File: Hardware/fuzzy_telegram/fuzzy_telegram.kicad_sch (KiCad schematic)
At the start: 1 part, among them U1 STM32MP157DAB1

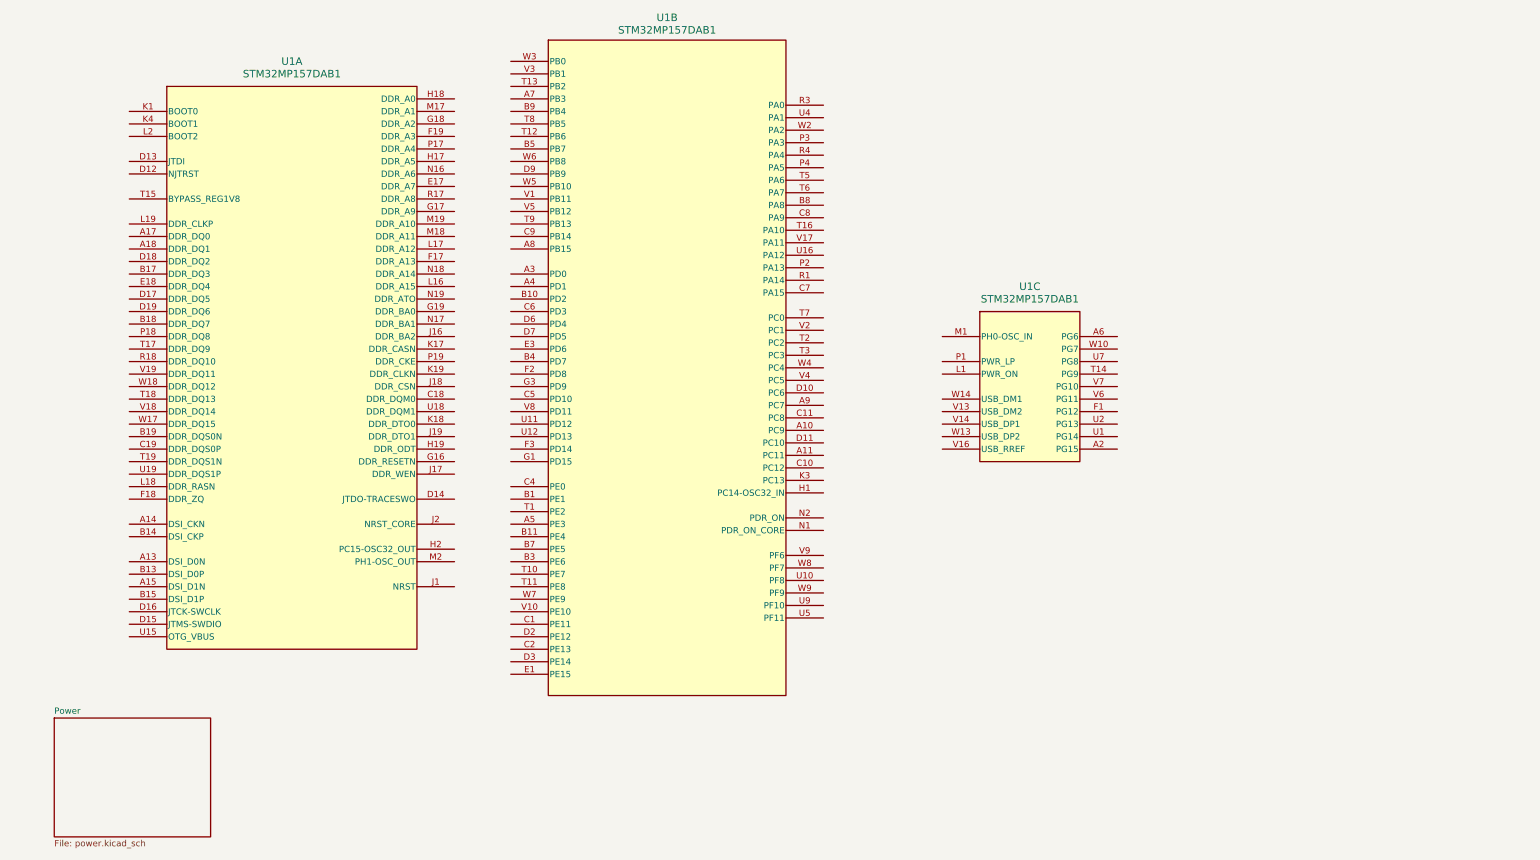
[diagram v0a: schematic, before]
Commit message: start on DDR3L schematic
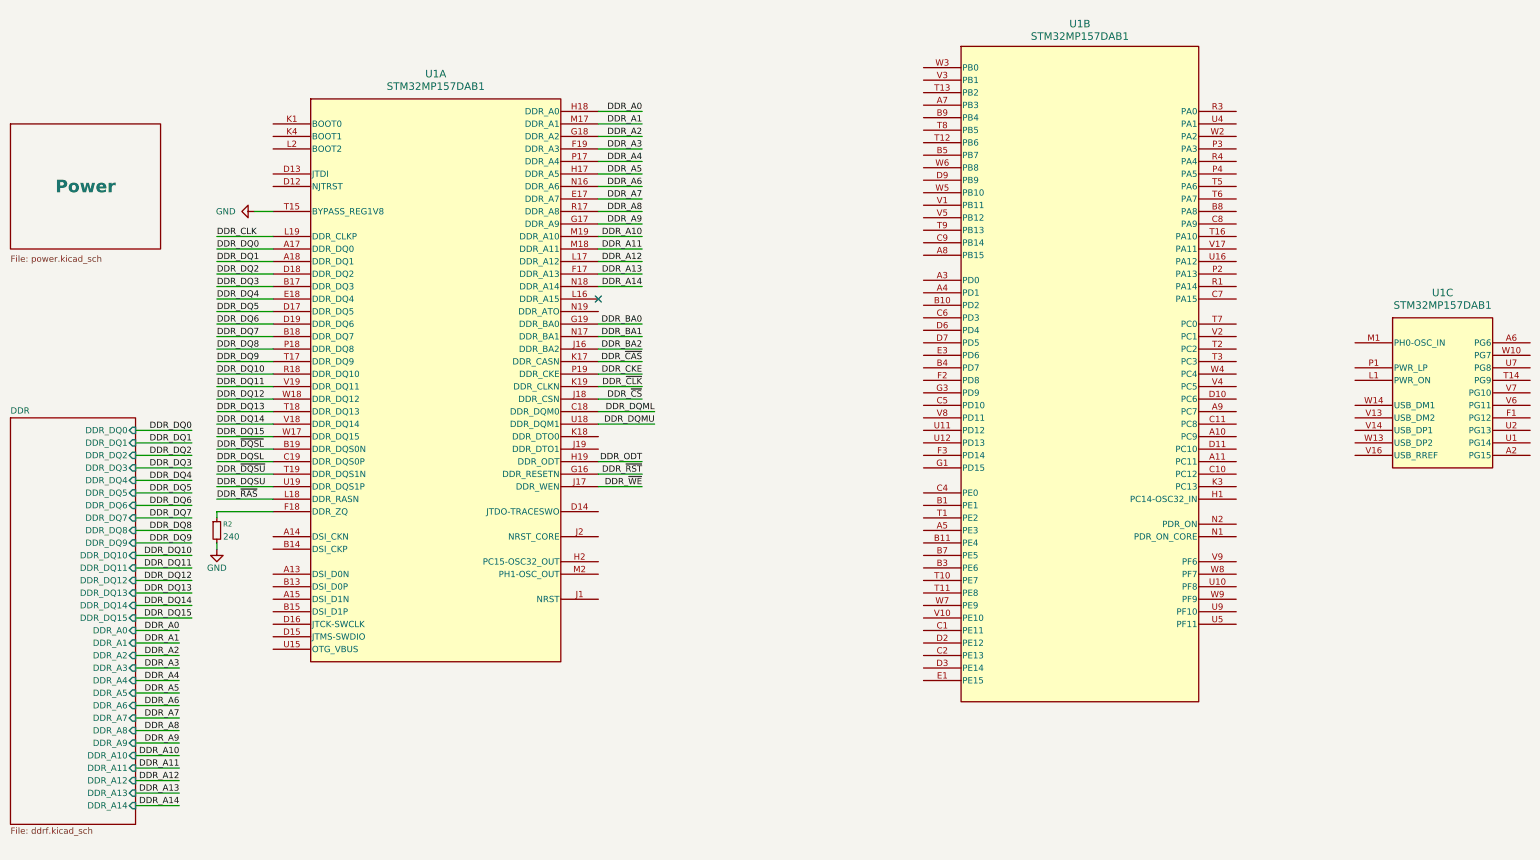
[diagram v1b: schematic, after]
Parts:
- added R2: 240, symbol Device:R_Small
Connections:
- net DDR_DQ0: now reaches U1.A17 (DDR_DQ0)
- net DDR_DQ1: now reaches U1.A18 (DDR_DQ1)
- net DDR_DQ3: now reaches U1.B17 (DDR_DQ3)
- net DDR_DQ7: now reaches U1.B18 (DDR_DQ7)
- net DDR_~{DQSL}: now reaches U1.B19 (DDR_DQS0N)
- net DDR_DQML: now reaches U1.C18 (DDR_DQM0)
- net DDR_DQSL: now reaches U1.C19 (DDR_DQS0P)
- net DDR_DQ5: now reaches U1.D17 (DDR_DQ5)
- net DDR_DQ2: now reaches U1.D18 (DDR_DQ2)
- net DDR_DQ6: now reaches U1.D19 (DDR_DQ6)
- net DDR_A7: now reaches U1.E17 (DDR_A7)
- net DDR_DQ4: now reaches U1.E18 (DDR_DQ4)
- net DDR_A13: now reaches U1.F17 (DDR_A13)
- net at U1.F18 (DDR_ZQ): now also R2.1
- net DDR_A3: now reaches U1.F19 (DDR_A3)
- net DDR_~{RST}: now reaches U1.G16 (DDR_RESETN)
- net DDR_A9: now reaches U1.G17 (DDR_A9)
- net DDR_A2: now reaches U1.G18 (DDR_A2)
- net DDR_BA0: now reaches U1.G19 (DDR_BA0)
- net DDR_A5: now reaches U1.H17 (DDR_A5)
- net DDR_A0: now reaches U1.H18 (DDR_A0)
- net DDR_ODT: now reaches U1.H19 (DDR_ODT)
- net DDR_BA2: now reaches U1.J16 (DDR_BA2)
- net DDR_~{WE}: now reaches U1.J17 (DDR_WEN)
- net DDR_~{CS}: now reaches U1.J18 (DDR_CSN)
- net DDR_~{CAS}: now reaches U1.K17 (DDR_CASN)
- net DDR_~{CLK}: now reaches U1.K19 (DDR_CLKN)
- net DDR_A12: now reaches U1.L17 (DDR_A12)
- net DDR_~{RAS}: now reaches U1.L18 (DDR_RASN)
- net DDR_CLK: now reaches U1.L19 (DDR_CLKP)
- net DDR_A1: now reaches U1.M17 (DDR_A1)
- net DDR_A11: now reaches U1.M18 (DDR_A11)
- net DDR_A10: now reaches U1.M19 (DDR_A10)
- net DDR_A6: now reaches U1.N16 (DDR_A6)
- net DDR_BA1: now reaches U1.N17 (DDR_BA1)
- net DDR_A14: now reaches U1.N18 (DDR_A14)
- net DDR_A4: now reaches U1.P17 (DDR_A4)
- net DDR_DQ8: now reaches U1.P18 (DDR_DQ8)
- net DDR_CKE: now reaches U1.P19 (DDR_CKE)
- net DDR_A8: now reaches U1.R17 (DDR_A8)
- net DDR_DQ10: now reaches U1.R18 (DDR_DQ10)
- net GND: now reaches U1.T15 (BYPASS_REG1V8)
- net GND: now also R2.2
- net DDR_DQ9: now reaches U1.T17 (DDR_DQ9)
- net DDR_DQ13: now reaches U1.T18 (DDR_DQ13)
- net DDR_~{DQSU}: now reaches U1.T19 (DDR_DQS1N)
- net DDR_DQMU: now reaches U1.U18 (DDR_DQM1)
- net DDR_DQSU: now reaches U1.U19 (DDR_DQS1P)
- net DDR_DQ14: now reaches U1.V18 (DDR_DQ14)
- net DDR_DQ11: now reaches U1.V19 (DDR_DQ11)
- net DDR_DQ15: now reaches U1.W17 (DDR_DQ15)
- net DDR_DQ12: now reaches U1.W18 (DDR_DQ12)
- no-connect marks 0 -> 1
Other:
- added sheet DDR (ddrf.kicad_sch)
- moved on the sheet: U1B, U1C
